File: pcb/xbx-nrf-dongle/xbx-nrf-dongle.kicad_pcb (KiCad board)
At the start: 2 copper layers, 59.8 x 82.3 mm, 57 parts, among them J1 SWD, J2 UART, J3 16P-USBC-RECEPTACLE, SW1 SW_Push, SW2 SW_Push, SW3 SW_SPDT, U1 LDS3985M33R_SOT23, U2 USBLC6-2SC6, U3 MDBT50Q-U1MV2, Y1 32.768kHz

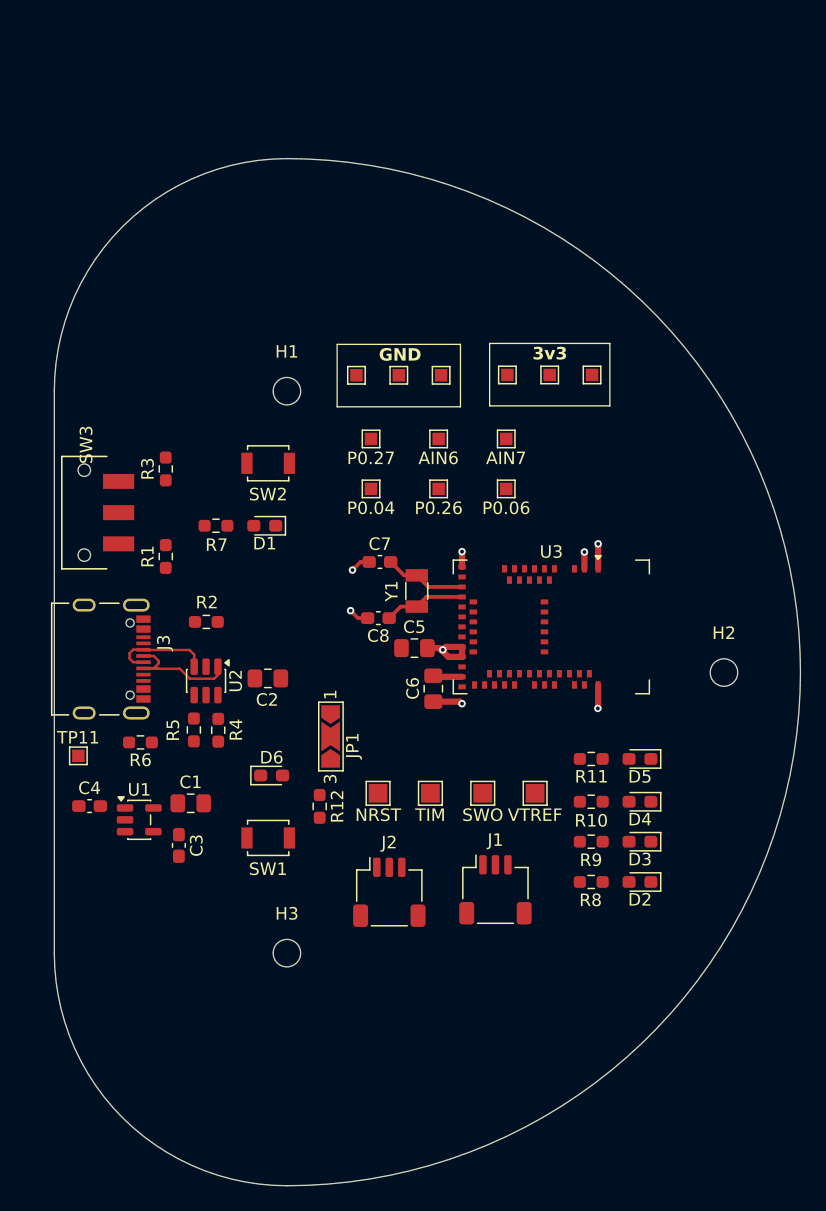
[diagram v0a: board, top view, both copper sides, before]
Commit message: Change board shape, reposition components. Pre-routing commit
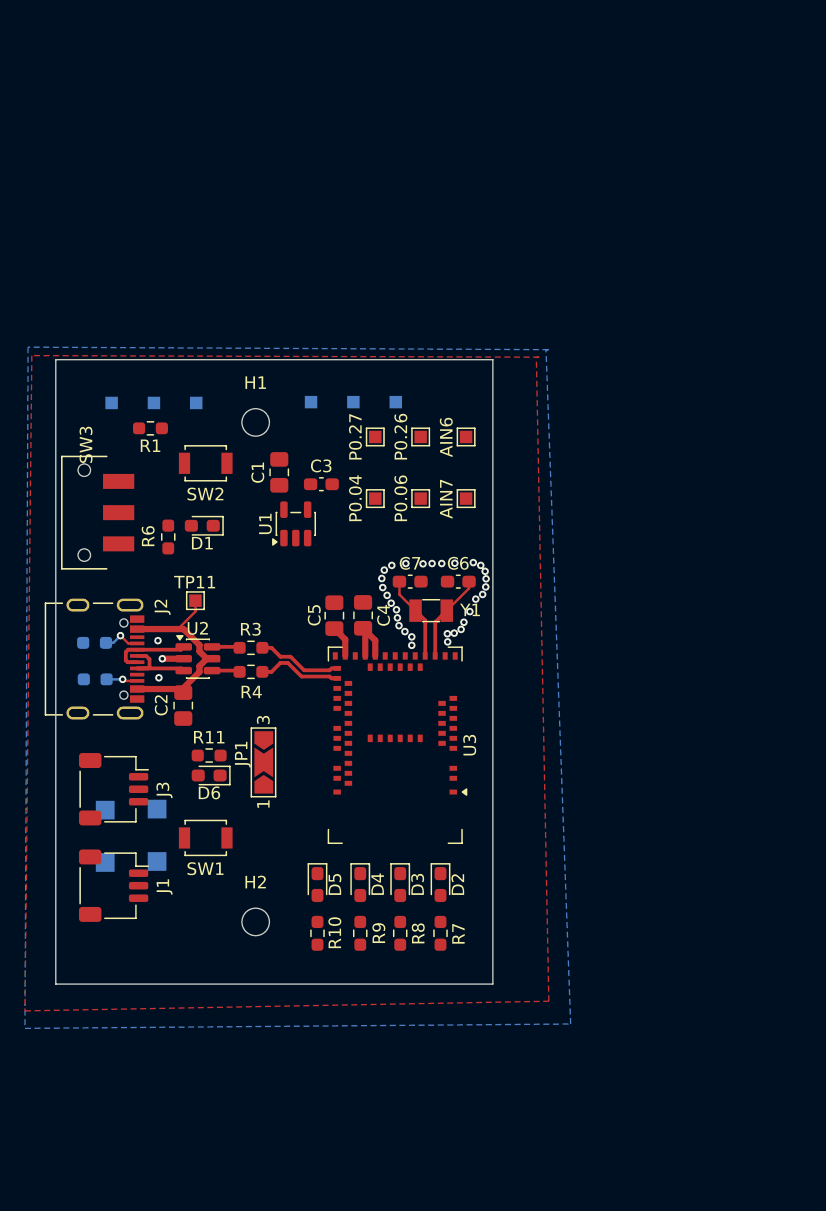
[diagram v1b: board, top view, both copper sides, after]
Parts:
- removed the C4 at (70.4, 97.8)
- removed the H2 at (121.2, 87.1)
- removed the R3 at (76.5, 70.8)
- R2, TP1, TP10, TP2, TP3, TP4, TP5, TP6, TP7, TP8, TP9: moved to B.Cu
- R5: renamed from R6; moved to B.Cu
- moved C3 31.1 mm to (89.0, 72.0), turned to 0 degrees
- moved TP2 30.8 mm to (75.8, 102.2), turned to -90 degrees
- moved J1 30.6 mm to (72.3, 104.1), turned to -90 degrees
- moved D5 27.7 mm to (88.7, 104.0), turned to -90 degrees
- moved C1 27.4 mm to (85.6, 71.0), turned to 90 degrees
- moved U1 26.8 mm to (86.9, 75.2), turned to 90 degrees
- moved TP4 26.6 mm to (71.7, 102.3), turned to -90 degrees
- moved TP3 26.1 mm to (75.8, 98.0), turned to -90 degrees
- moved R10 26.0 mm to (88.7, 107.9), turned to 90 degrees
- moved J3 23.6 mm to (72.3, 96.4), turned to -90 degrees
- moved D4 23.4 mm to (92.1, 104.0), turned to -90 degrees
- moved TP1 21.9 mm to (71.7, 98.1), turned to -90 degrees
- moved R9 21.3 mm to (92.1, 107.9), turned to 90 degrees
- moved TP5 19.7 mm to (75.6, 65.5)
- moved TP6 19.7 mm to (72.2, 65.5)
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- renumbered C5 to C4, C6 to C5, C7 to C6, C8 to C7, H3 to H2, J3 to J2, J2 to J3, R11 to R10, R12 to R11, R4 to R3, R5 to R4, R7 to R6, R8 to R7, R9 to R8, R10 to R9
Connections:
- net Net-(U3-P0.00) renamed /XL1
- net Net-(U3-P0.01) renamed /XL2
- R1 pad 1: +3V3 -> GND
- R3 pad 1: /D+ -> /D-
- R4 pad 2: /D- -> /D+
- SW3 pad 1: Net-(R3-Pad1) -> unconnected-(SW3-Pad1)
- U2 pad 1: /EXT_D+ -> /EXT_D-
- U2 pad 3: /EXT_D- -> /EXT_D+
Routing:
- net VBUS: track 2.34 -> 19.6 mm
- net GND: track 12.1 -> 1.71 mm, vias 7 -> 33
- net /D+: track 0.00 -> 6.80 mm
- net /D-: track 0.00 -> 6.80 mm
- net /EXT_D+: track 10.3 -> 6.59 mm
- net Net-(J2-CC1): track 0.00 -> 2.99 mm, vias 0 -> 1
- net Net-(J2-CC2): track 0.00 -> 2.50 mm, vias 0 -> 1
- net Net-(R4-Pad1): track 0.00 -> 2.24 mm
- net Net-(R3-Pad2): track 0.00 -> 2.23 mm
- net /EXT_D-: track 9.24 -> 8.09 mm
- net +3V3: track 5.59 -> 4.90 mm, vias 1 -> 0
- net /XL1: track 6.54 -> 7.07 mm
- added copper zone on B.Cu, net GND
- added copper zone on F.Cu, net GND
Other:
- board size 59.8 x 82.3 mm -> 35 x 50 mm
- board text added: "ANTENNA ZONE"

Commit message: Dongle PCB Rev1 complete
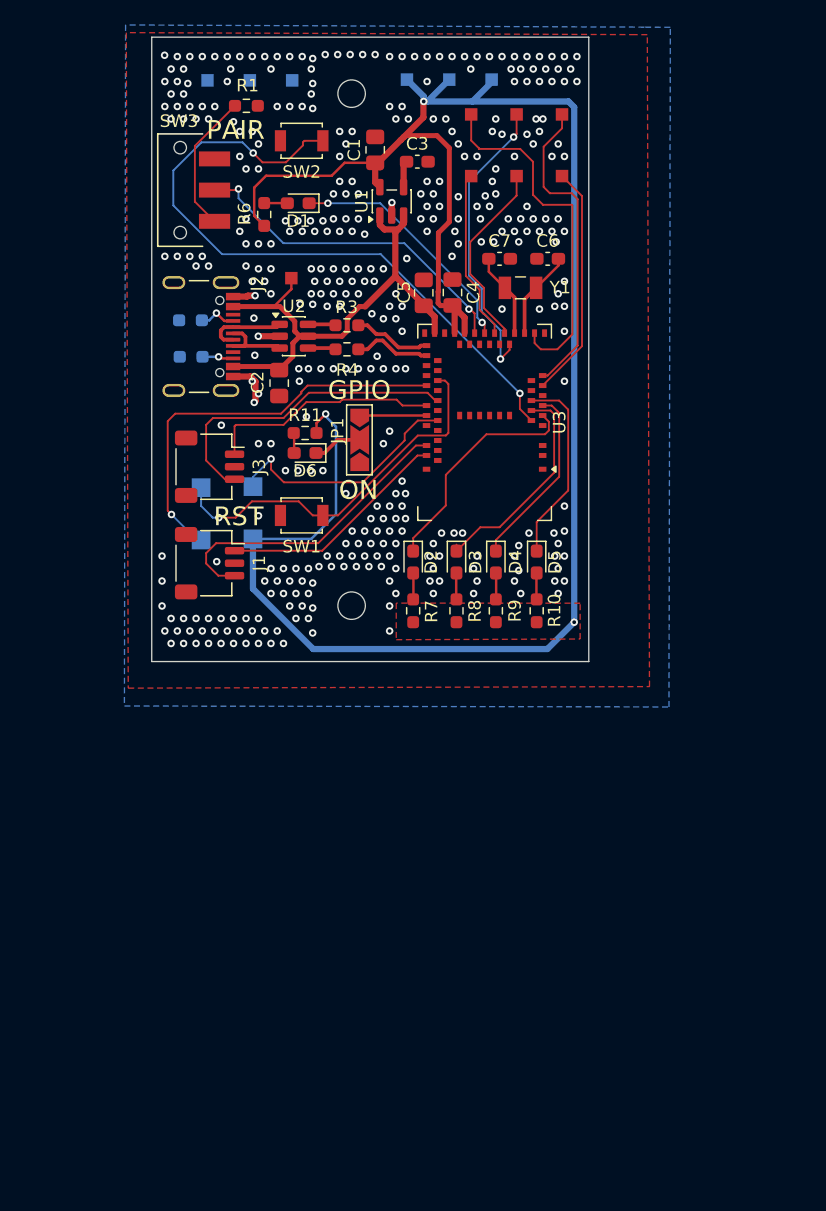
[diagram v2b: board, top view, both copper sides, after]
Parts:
- J2: footprint usbc-16p-receptacle-amphenol:USB_C_Receptacle_16P_Amphenol_10155435-00011LF -> xbx-nrf-lib:USB_C_Receptacle_16P_Amphenol_10155435-00011LF
- JP1: footprint Jumper:SolderJumper-3_P2.0mm_Open_TrianglePad1.0x1.5mm_NumberLabels -> xbx-nrf-lib:SolderJumper-3_P2.0mm_Open_TrianglePad1.0x1.5mm_NumberLabels
- R1: value 10k -> 1k
- TP1, TP2, TP3, TP4: footprint TestPoint:TestPoint_Pad_1.5x1.5mm -> xbx-nrf-lib:TestPoint_Pad_1.5x1.5mm-NoSilkscreen
- TP10, TP11, TP12, TP13, TP14, TP15, TP16, TP17, TP5, TP6, TP7, TP8, TP9: footprint TestPoint:TestPoint_Pad_1.0x1.0mm -> xbx-nrf-lib:TestPoint_Pad_1.0x1.0mm-NoSilkscreen
- U3: footprint RF_Module:Raytac_MDBT50Q -> xbx-nrf-lib:Raytac_MDBT50Q
- Y1: footprint Crystal:Crystal_SMD_3215-2Pin_3.2x1.5mm -> xbx-nrf-lib:Crystal_SMD_3215-2Pin_3.2x1.5mm
- moved D5 31.2 mm to (106.2, 78.2)
- moved R10 31.2 mm to (106.2, 82.1)
- moved TP14 28.2 mm to (104.6, 47.3)
- moved D4 28.0 mm to (103.0, 78.2)
- moved R9 28.0 mm to (103.0, 82.1)
- moved H1 27.4 mm to (91.4, 40.7)
- moved J3 26.9 mm to (80.0, 70.6)
- moved TP3 26.9 mm to (83.5, 72.2)
- moved C1 26.9 mm to (93.3, 45.2)
- moved C2 26.9 mm to (85.6, 63.9)
- moved R3 26.9 mm to (91.0, 59.2)
- moved R6 26.9 mm to (84.4, 50.4)
- moved TP10 26.9 mm to (95.8, 39.6)
- moved TP5 26.9 mm to (83.3, 39.6)
- moved TP6 26.9 mm to (79.9, 39.6)
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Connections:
- U3 pad 10: /PWR_LED -> unconnected-(U3-P0.29-Pad10)
- U3 pad 11: /PAIR_LED -> unconnected-(U3-P0.02-Pad11)
- U3 pad 24: unconnected-(U3-P0.08-Pad24) -> /PAIR_LED
- U3 pad 26: unconnected-(U3-P1.09-Pad26) -> /MODE_SW
- U3 pad 4: /MODE_SW -> unconnected-(U3-P1.11-Pad4)
- U3 pad 46: unconnected-(U3-P0.22-Pad46) -> /PWR_LED
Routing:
- net +3V3: track 4.90 -> 157.5 mm, vias 0 -> 3
- net /PAIR_SW: track 0.00 -> 53.8 mm, vias 0 -> 2
- net /TIMING_PIN: track 0.00 -> 32.8 mm, vias 0 -> 1
- net /NRST: track 0.00 -> 30.4 mm, vias 0 -> 1
- net /P0.27: track 0.00 -> 28.8 mm
- net /MODE_SW: track 0.00 -> 27.1 mm, vias 0 -> 2
- net /DBG_TX: track 0.00 -> 25.6 mm
- net /AIN6: track 0.00 -> 25.1 mm
- net /SWDIO: track 0.00 -> 24.7 mm
- net /P0.26: track 0.00 -> 23.7 mm, vias 0 -> 2
- net VBUS: track 19.6 -> 40.8 mm
- net /SWO: track 0.00 -> 19.8 mm, vias 0 -> 1
- net /PAIR_LED: track 0.00 -> 19.6 mm, vias 0 -> 2
- net /AIN7: track 0.00 -> 18.7 mm
- net /DBG_RX: track 0.00 -> 18.7 mm
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- added copper zone on F.Cu, net +3V3
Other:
- board text added: "GPIO"
- board text added: "HID"
- board text added: "ON"
- board text added: "PAIR"
- board text added: "RST"
- board text added: "XINPUT"
